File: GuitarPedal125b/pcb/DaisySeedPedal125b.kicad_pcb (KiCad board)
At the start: 4 copper layers, 60 x 94 mm, 79 parts, among them J1 Barrel_Jack_Switch, J2 AUDIO_IN_TRS, J3 AUDIO_OUT_TRS, J4 MIDI IN JACK, J5 MIDI OUT JACK, K1 G6K-2, K2 G6K-2, Q1 SS8050, U1 LD1117S50TR_SOT223, U2 PDS1-S5-S5-M, U3 MCP6004, U4 OPA1652AID, U5 H11L1, U6 OLED_DISPLAY_SSD1306_SPI

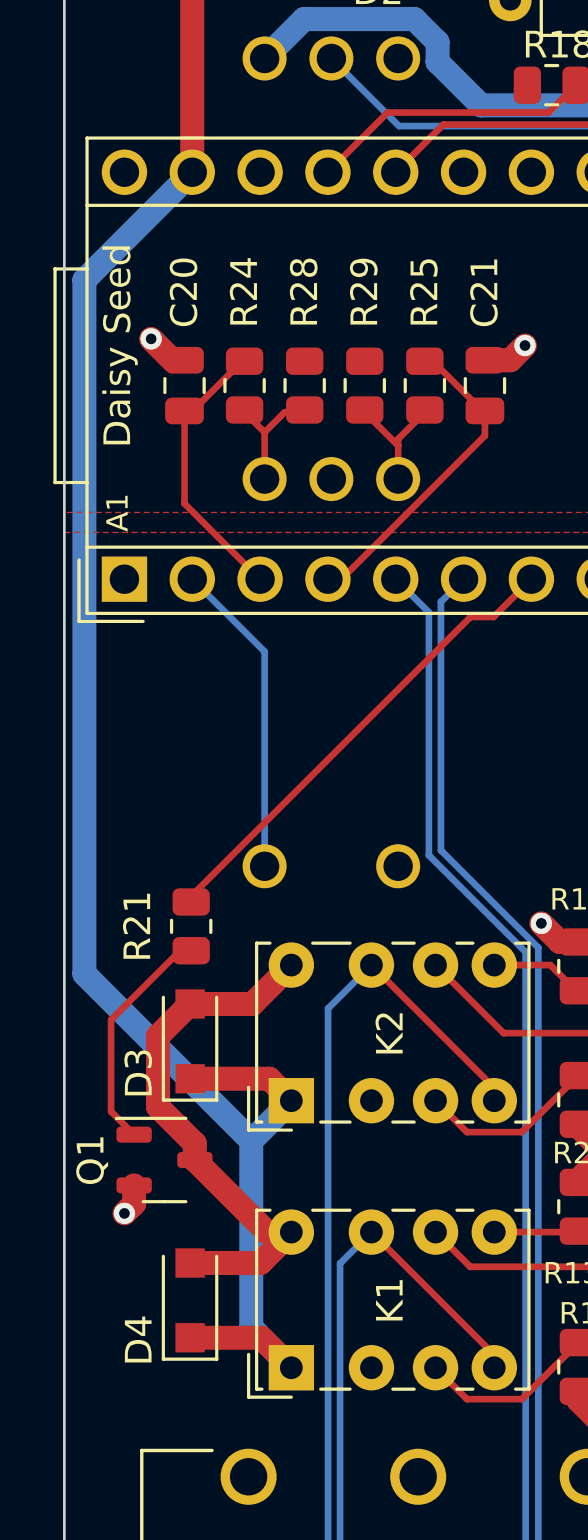
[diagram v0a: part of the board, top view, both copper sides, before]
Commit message: Updated PCB to use 5v power for the relay instead of 9v
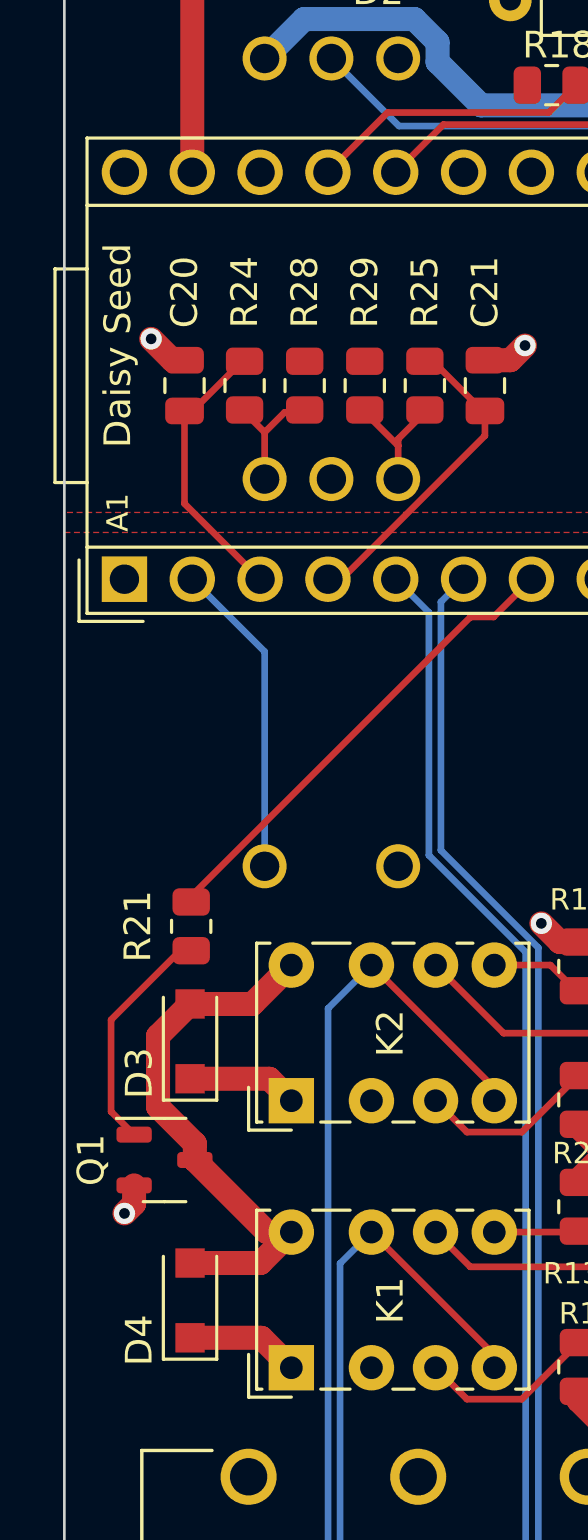
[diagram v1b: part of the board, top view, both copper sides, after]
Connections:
- D3 pad 1: +9V -> +5V_ISOLATED_POWER
- D4 pad 1: +9V -> +5V_ISOLATED_POWER
- K1 pad 1: +9V -> +5V_ISOLATED_POWER
- K2 pad 1: +9V -> +5V_ISOLATED_POWER
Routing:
- net +9V: track 113.8 -> 53.6 mm
- net +5V_ISOLATED_POWER: track 49.4 -> 57.8 mm
